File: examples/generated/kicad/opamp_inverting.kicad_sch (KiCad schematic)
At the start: 6 parts

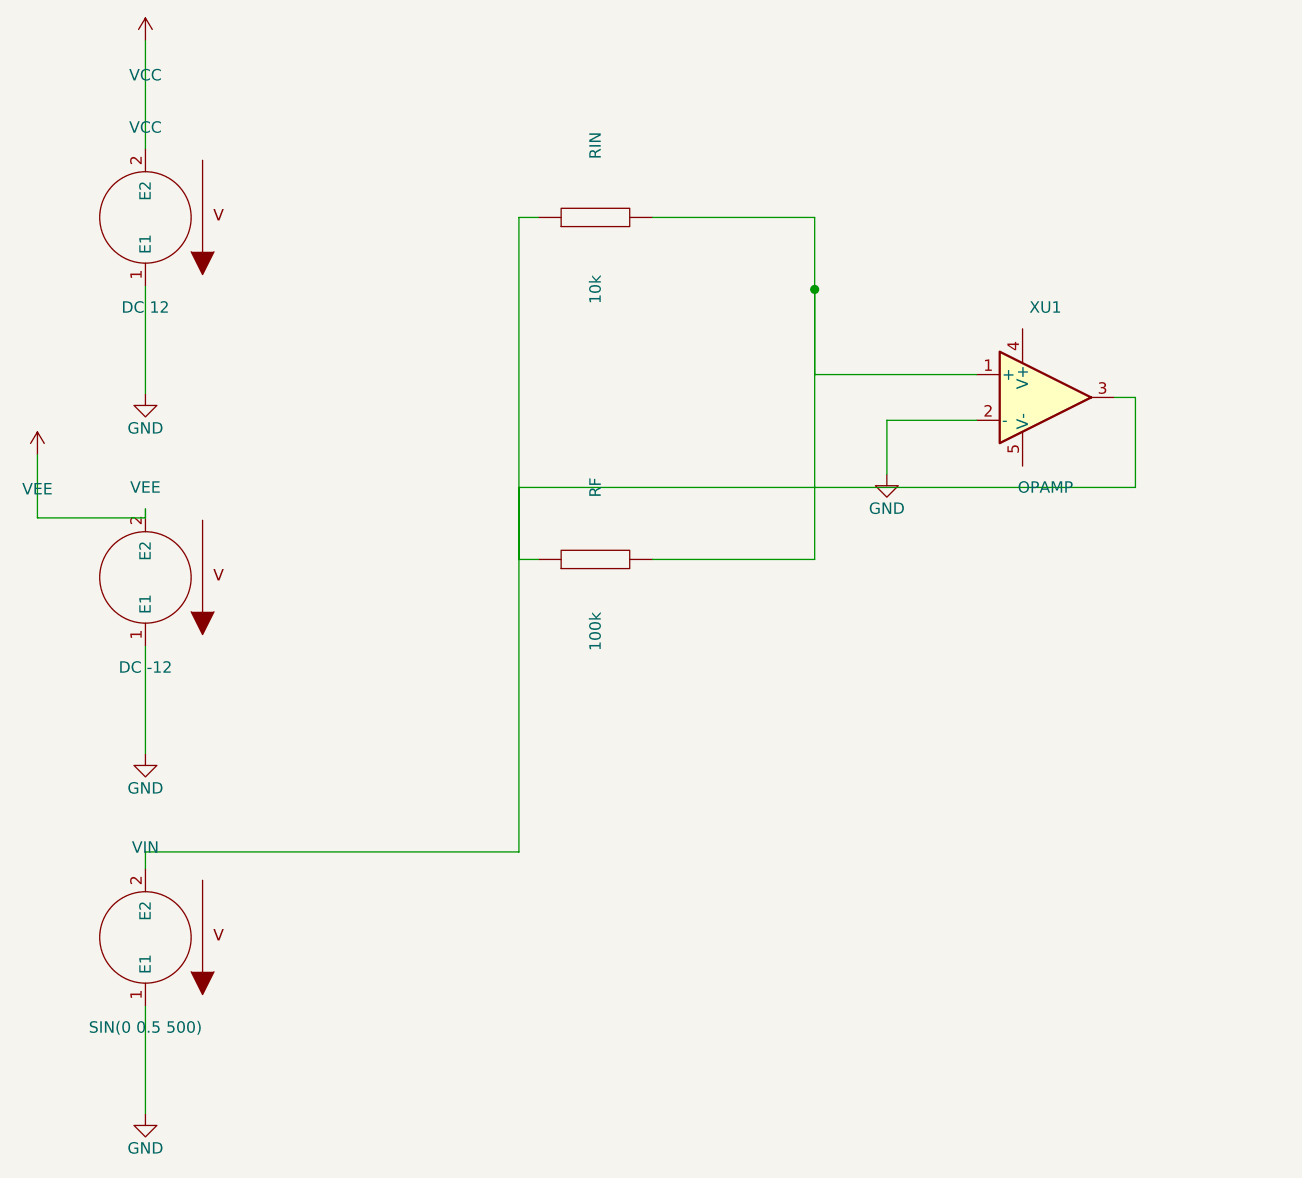
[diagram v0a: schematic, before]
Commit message: Attempt to fix more terminal issues.
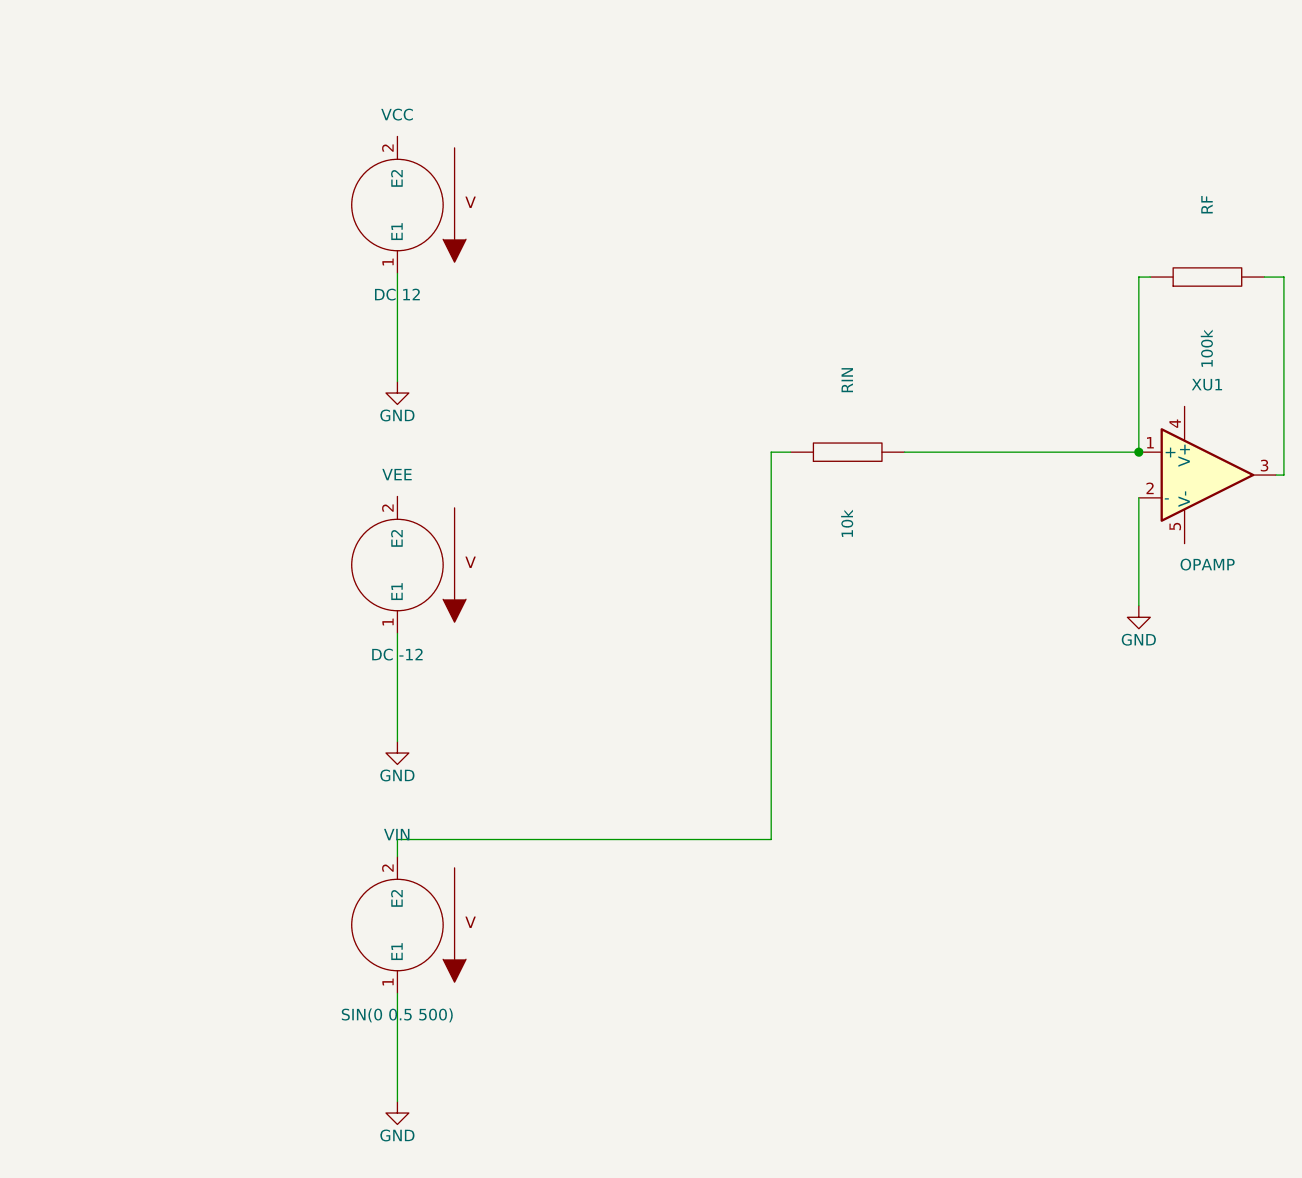
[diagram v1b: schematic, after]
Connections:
- net at RIN.2, XU1.1 (+): now also RF.1; no longer RF.2
- net at RIN.1, VIN.2 (E2): no longer RF.1, XU1.3
- net VCC: no longer names the net of VCC.2 (E2)
- net VEE: no longer names the net of VEE.2 (E2)
- new net: RF.2, XU1.3
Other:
- moved on the sheet: RF, RIN, VCC, VEE, VIN, XU1
